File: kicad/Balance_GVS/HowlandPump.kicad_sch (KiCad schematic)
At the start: 16 parts, among them J11 Conn_01x02_Pin, U11 LT1013DIP, U12 LT1013DIP

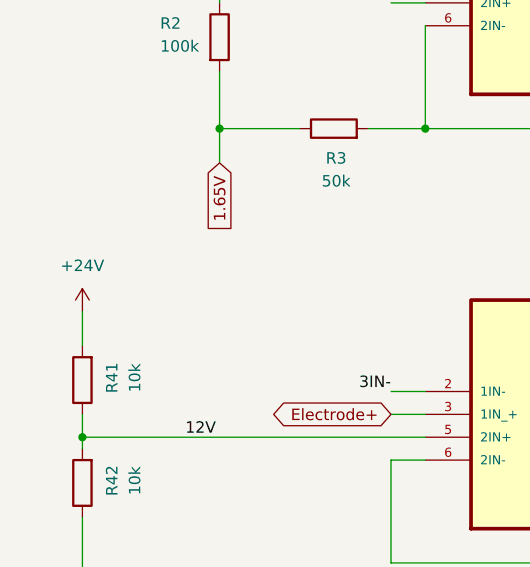
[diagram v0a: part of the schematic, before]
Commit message: I kinda popped off ngl. Main pcb almost done
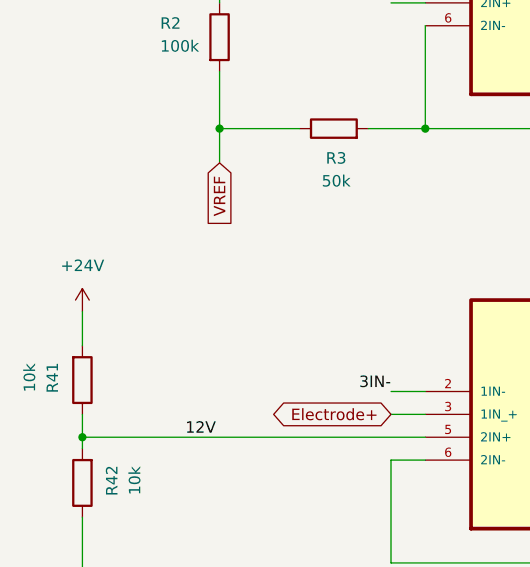
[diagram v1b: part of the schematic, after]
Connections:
- net 1.65V renamed VREF
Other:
- moved on the sheet: R41
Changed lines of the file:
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@@
-		)
-	)
-	(global_label "1.65V"
-		(shape input)
-		(at 71.12 104.14 270)
-		(fields_autoplaced yes)
-		(effects
-			(font
-				(size 1.27 1.27)
-			)
-			(justify right)
-		)
-		(property "Intersheetrefs" "${INTERSHEET_REFS}"
-			(at 71.12 112.4471 90)
-			(hide yes)
-			(show_name no)
-			(do_not_autoplace no)
-			(effects
-				(font
-					(size 1.27 1.27)
-				)
-				(justify right)
-			)
 		)
 	)
@@
 		)
 	)
+	(global_label "VREF"
+		(shape input)
+		(at 71.12 104.14 270)
+		(fields_autoplaced yes)
+		(effects
+			(font
+				(size 1.27 1.27)
+			)
+			(justify right)
+		)
+		(property "Intersheetrefs" "${INTERSHEET_REFS}"
+			(at 71.12 111.7214 90)
+			(hide yes)
+			(show_name no)
+			(do_not_autoplace no)
+			(effects
+				(font
+					(size 1.27 1.27)
+				)
+				(justify right)
+			)
+		)
+	)
 	(symbol
 		(lib_id "Device:R")
@@
 	(symbol
 		(lib_id "Device:R")
-		(at 55.88 128.27 180)
+		(at 55.88 128.27 0)
+		(mirror x)
 		(unit 1)
 		(body_style 1)
@@
 		(dnp no)
 		(property "Reference" "R41"
-			(at 59.182 128.016 90)
+			(at 52.578 128.016 90)
 			(show_name no)
 			(do_not_autoplace no)
@@
 		)
 		(property "Value" "10k"
-			(at 61.722 128.016 90)
+			(at 50.038 128.016 90)
 			(show_name no)
 			(do_not_autoplace no)
@@
 		)
 		(property "Footprint" "Resistor_SMD:R_0805_2012Metric_Pad1.20x1.40mm_HandSolder"
-			(at 57.658 128.27 90)
-			(hide yes)
-			(show_name no)
+			(at 54.102 128.27 90)
+			(hide yes)
+			(show_name no)
